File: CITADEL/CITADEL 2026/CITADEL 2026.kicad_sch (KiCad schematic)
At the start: 33 parts, among them J1 Vibration Motor, J2 Linear Actuator, U3 TJA1051T-3

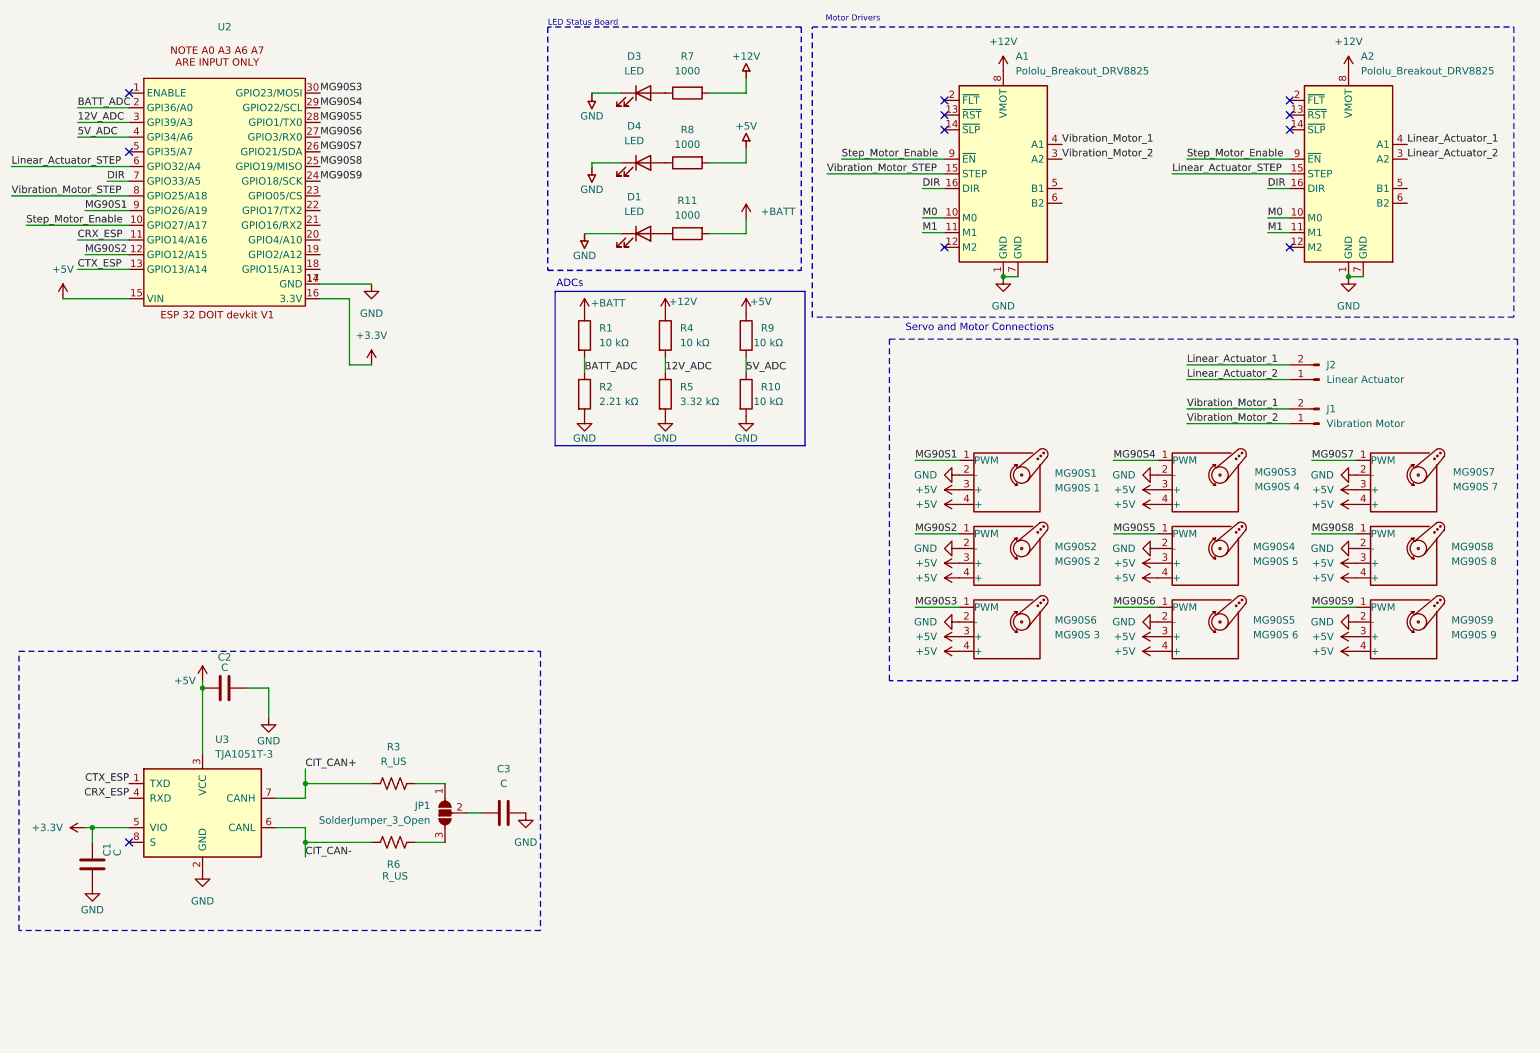
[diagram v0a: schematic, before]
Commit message: Updated Schematic
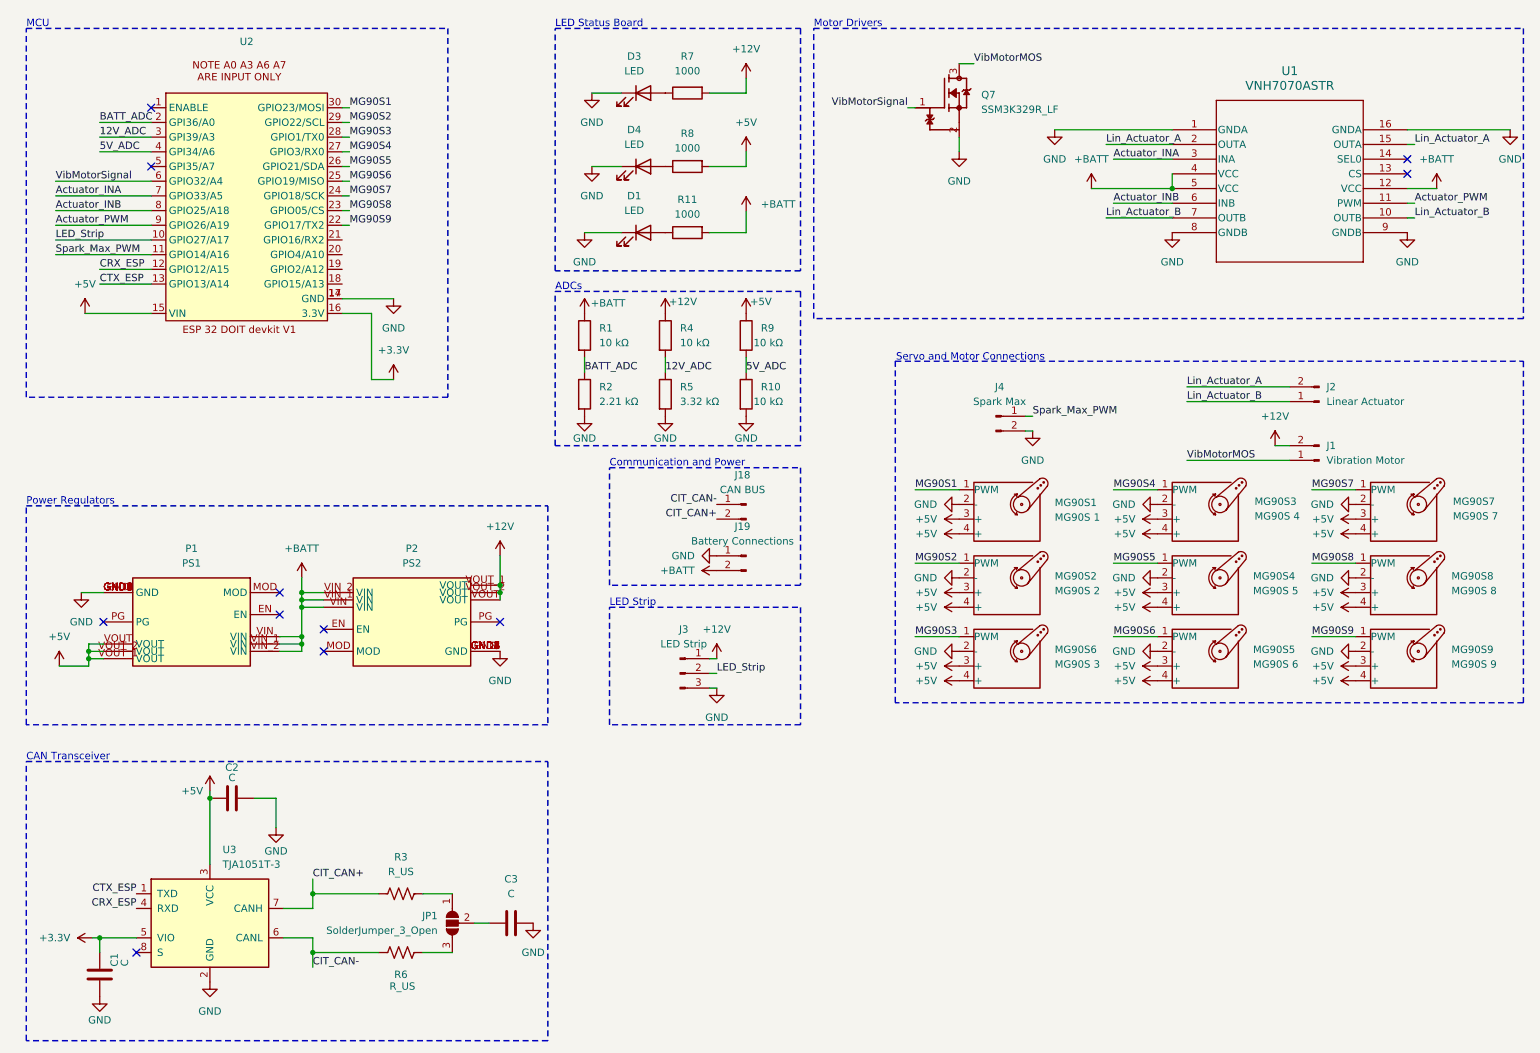
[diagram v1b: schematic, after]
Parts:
- removed A1, A2: Pololu_Breakout_DRV8825, Module:Pololu_Breakout-16_15.2x20.3mm, symbol Driver_Motor:Pololu_Breakout_DRV8825
- added J18: CAN BUS, Connector_AMASS:AMASS_XT30U-F_1x02_P5.0mm_Vertical, symbol Connector:Conn_01x02_Pin
- added J19: Battery Connections, Connector_AMASS:AMASS_XT60-M_1x02_P7.20mm_Vertical, symbol Connector:Conn_01x02_Pin
- added J3: LED Strip, Connector_JST:JST_EH_B3B-EH-A_1x03_P2.50mm_Vertical, symbol Connector:Conn_01x03_Pin
- added J4: Spark Max, Connector_JST:JST_EH_B2B-EH-A_1x02_P2.50mm_Vertical, symbol Connector:Conn_01x02_Pin
- added P1: PS1, Citadel:D24V15OF5, symbol Citadel-altium-import:root_2_Pololu_5V,_15A_Step-Down_Voltage_Regulator_D24V150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
- added P2: PS2, Citadel:D24V15OF5, symbol Citadel-altium-import:root_0_Pololu_12V,_15A_Step-Down_Voltage_Regulator_D24V15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
- added Q7: SSM3K329R_LF, Citadel:SSM3K329_LF, symbol Citadel-altium-import:root_0_SSM3K329R_LF
- added U1: VNH7070ASTR, Jayse_Footprints:SO_0ASTR_STM, symbol 2026-01-09_23-32-14:VNH7070ASTR
- MG90S1, MG90S2, MG90S3, MG90S4, MG90S5, MG90S6, MG90S7, MG90S8, MG90S9: footprint (none) -> Connector_Molex:Molex_Mini-Fit_Jr_5566-04A_2x02_P4.20mm_Vertical
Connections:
- net Vibration_Motor_1 is gone; now on net +12V: J1.2 (Pin_2)
- net +12V: now also J3.1 (Pin_1), P2.VOUT, P2.VOUT_1 (VOUT), P2.VOUT_2 (VOUT)
- net +5V: now also P1.VOUT, P1.VOUT_1 (VOUT), P1.VOUT_2 (VOUT)
- net +BATT: now also J19.2 (Pin_2), P1.VIN, P1.VIN_1 (VIN), P1.VIN_2 (VIN), P2.VIN, P2.VIN_1 (VIN), P2.VIN_2 (VIN), U1.12 (VCC), U1.4 (VCC), U1.5 (VCC)
- net CIT_CAN+: now also J18.2 (Pin_2)
- net CIT_CAN-: now also J18.1 (Pin_1)
- net CRX_ESP: now also U2.12 (GPIO12/A15); no longer U2.11 (GPIO14/A16)
- net GND: now also J19.1 (Pin_1), J3.3 (Pin_3), J4.2 (Pin_2), P1.GND, P1.GND1 (GND), P1.GND2 (GND), P1.GND3 (GND), P1.GND4 (GND), P1.GND5 (GND), P1.GND6 (GND), P1.GND7 (GND), P2.GND, P2.GND1 (GND), P2.GND2 (GND), P2.GND3 (GND), P2.GND4 (GND), P2.GND5 (GND), P2.GND6 (GND), P2.GND7 (GND), Q7.2, U1.1 (GNDA), U1.16 (GNDA), U1.8 (GNDB), U1.9 (GNDB)
- net MG90S1: now also U2.30 (GPIO23/MOSI); no longer U2.9 (GPIO26/A19)
- net MG90S2: now also U2.29 (GPIO22/SCL); no longer U2.12 (GPIO12/A15)
- net MG90S3: now also U2.28 (GPIO1/TX0); no longer U2.30 (GPIO23/MOSI)
- net MG90S4: now also U2.27 (GPIO3/RX0); no longer U2.29 (GPIO22/SCL)
- net MG90S5: now also U2.26 (GPIO21/SDA); no longer U2.28 (GPIO1/TX0)
- net MG90S6: now also U2.25 (GPIO19/MISO); no longer U2.27 (GPIO3/RX0)
- net MG90S7: now also U2.24 (GPIO18/SCK); no longer U2.26 (GPIO21/SDA)
- net MG90S8: now also U2.23 (GPIO05/CS); no longer U2.25 (GPIO19/MISO)
- net MG90S9: now also U2.22 (GPIO17/TX2); no longer U2.24 (GPIO18/SCK)
- net DIR renamed Actuator_INA
- net Actuator_INA: now also U1.3 (INA)
- net Linear_Actuator_1 renamed Lin_Actuator_A
- net Lin_Actuator_A: now also U1.15 (OUTA), U1.2 (OUTA)
- net Linear_Actuator_2 renamed Lin_Actuator_B
- net Lin_Actuator_B: now also U1.10 (OUTB), U1.7 (OUTB)
- net Linear_Actuator_STEP renamed VibMotorSignal
- net VibMotorSignal: now also Q7.1
- net Step_Motor_Enable renamed LED_Strip
- net LED_Strip: now also J3.2 (Pin_2)
- net Vibration_Motor_2 renamed VibMotorMOS
- net VibMotorMOS: now also Q7.3
- net Vibration_Motor_STEP renamed Actuator_INB
- net Actuator_INB: now also U1.6 (INB)
- new net Actuator_PWM: U1.11 (PWM), U2.9 (GPIO26/A19)
- new net Spark_Max_PWM: J4.1 (Pin_1), U2.11 (GPIO14/A16)
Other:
- note added: "CAN Transceiver"
- note added: "Communication and Power"
- note added: "LED Strip"
- note added: "MCU"
- note added: "Power Regulators"
- moved on the sheet: C1, C2, C3, D4, J1, J2, JP1, MG90S1, MG90S2, MG90S3, MG90S4, MG90S5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
